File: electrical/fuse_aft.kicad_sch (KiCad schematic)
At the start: 4 parts, among them U1 GSU25, U2 GTX45R, U4 GSA 28 PITCH, U8 ESSENTIAL

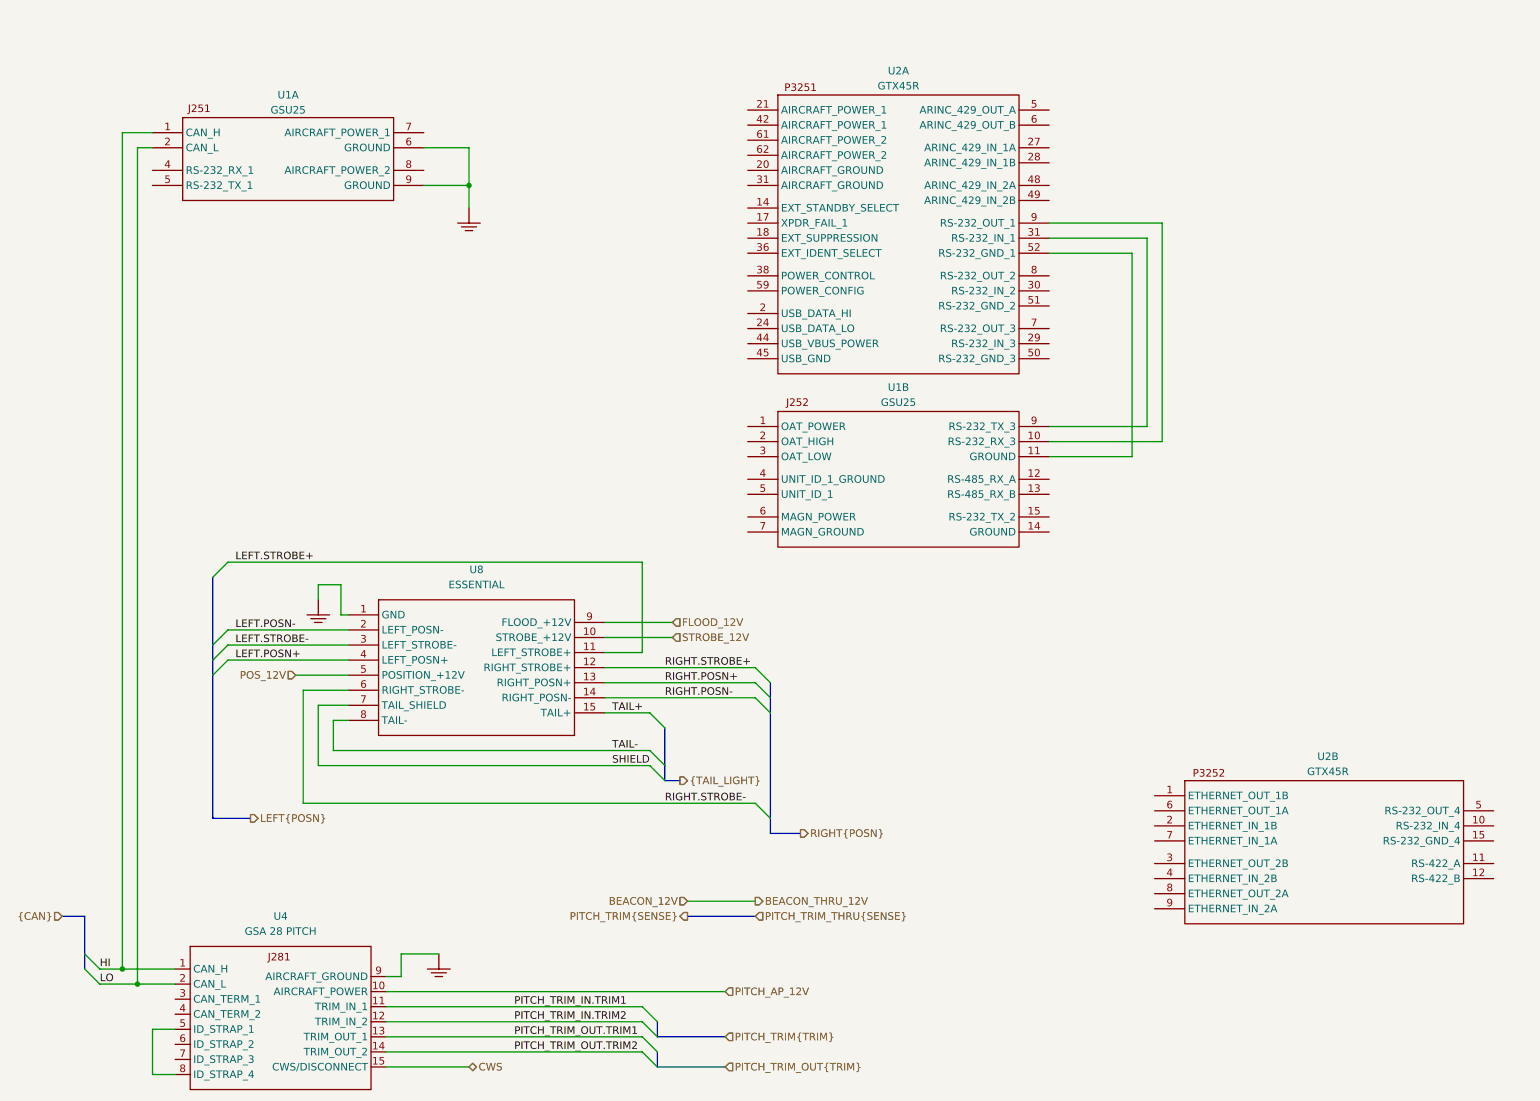
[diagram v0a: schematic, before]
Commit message: 🎮 Working on electrical schematic
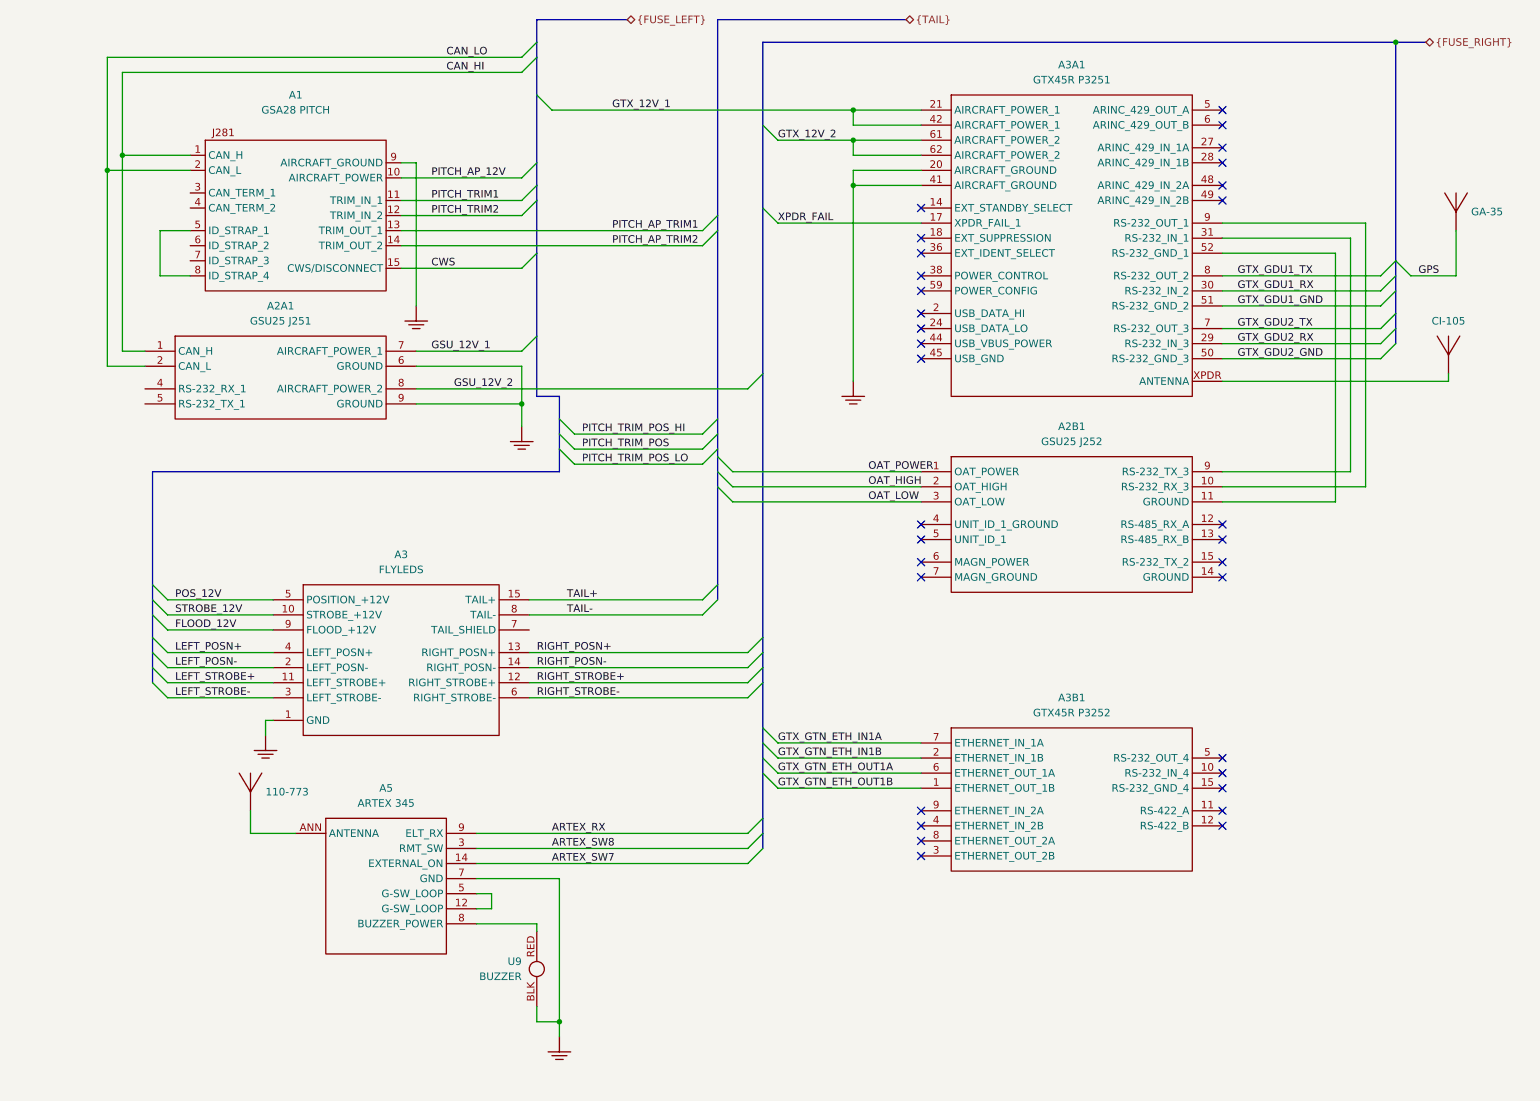
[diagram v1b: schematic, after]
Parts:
- removed U1: GSU25, symbol Garmin:GSU25
- removed U2: GTX45R, symbol Garmin:GTX45R
- removed U8: ESSENTIAL, symbol FlyLeds:ESSENTIAL_CONTROLLER
- added A2A1: GSU25 J251, symbol Garmin:GSU25_J251
- added A2B1: GSU25 J252, symbol Garmin:GSU25_J252
- added A3: FLYLEDS, symbol FlyLeds:ESSENTIAL_CONTROLLER
- added A3A1: GTX45R P3251, symbol Garmin:GTX45R_P3251
- added A3B1: GTX45R P3252, symbol Garmin:GTX45R_P3252
- added A5: ARTEX 345, symbol Misc:ARTEX345
- added A6: CI-105, symbol Misc:ANTENNA
- added A7: GA-35, symbol Misc:ANTENNA
- added A8: 110-773, symbol Misc:ANTENNA
- added U9: BUZZER, symbol Misc:BUZZER
- A1: renamed from U4; value GSA 28 PITCH -> GSA28 PITCH
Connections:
- net FLOOD_12V: now also A3.9 (FLOOD_+12V)
- net GND: now also A2A1.6 (GROUND), A2A1.9 (GROUND), A3.1 (GND), A3A1.20 (AIRCRAFT_GROUND), A3A1.41 (AIRCRAFT_GROUND), A5.7 (GND), U9.BLK
- net POS_12V: now also A3.5 (POSITION_+12V)
- net STROBE_12V: now also A3.10 (STROBE_+12V)
- net TAIL+: now also A3.15 (TAIL+)
- net TAIL-: now also A3.8 (TAIL-)
- net HI renamed CAN_HI
- net CAN_HI: now also A2A1.1 (CAN_H)
- net LO renamed CAN_LO
- net CAN_LO: now also A2A1.2 (CAN_L)
- net PITCH_TRIM_IN.TRIM1 renamed PITCH_TRIM1
- net PITCH_TRIM_IN.TRIM2 renamed PITCH_TRIM2
- net PITCH_TRIM_OUT.TRIM1 renamed PITCH_AP_TRIM1
- net PITCH_TRIM_OUT.TRIM2 renamed PITCH_AP_TRIM2
- new net: A3A1.XPDR (ANTENNA), A6. (SIGNAL)
- new net: A2B1.9 (RS-232_TX_3), A3A1.31 (RS-232_IN_1)
- new net: A2B1.11 (GROUND), A3A1.52 (RS-232_GND_1)
- new net: A2B1.10 (RS-232_RX_3), A3A1.9 (RS-232_OUT_1)
- new net: A5.12 (G-SW_LOOP), A5.5 (G-SW_LOOP)
- new net: A5.8 (BUZZER_POWER), U9.RED
- new net: A5.ANN (ANTENNA), A8. (SIGNAL)
- new net ARTEX_RX: A5.9 (ELT_RX)
- new net ARTEX_SW7: A5.14 (EXTERNAL_ON)
- new net ARTEX_SW8: A5.3 (RMT_SW)
- new net GPS: A7. (SIGNAL)
- new net GSU_12V_1: A2A1.7 (AIRCRAFT_POWER_1)
- new net GSU_12V_2: A2A1.8 (AIRCRAFT_POWER_2)
- new net GTX_12V_1: A3A1.21 (AIRCRAFT_POWER_1), A3A1.42 (AIRCRAFT_POWER_1)
- new net GTX_12V_2: A3A1.61 (AIRCRAFT_POWER_2), A3A1.62 (AIRCRAFT_POWER_2)
- new net GTX_GDU1_GND: A3A1.51 (RS-232_GND_2)
- new net GTX_GDU1_RX: A3A1.30 (RS-232_IN_2)
- new net GTX_GDU1_TX: A3A1.8 (RS-232_OUT_2)
- new net GTX_GDU2_GND: A3A1.50 (RS-232_GND_3)
- new net GTX_GDU2_RX: A3A1.29 (RS-232_IN_3)
- new net GTX_GDU2_TX: A3A1.7 (RS-232_OUT_3)
- new net GTX_GTN_ETH_IN1A: A3B1.7 (ETHERNET_IN_1A)
- new net GTX_GTN_ETH_IN1B: A3B1.2 (ETHERNET_IN_1B)
- new net GTX_GTN_ETH_OUT1A: A3B1.6 (ETHERNET_OUT_1A)
- new net GTX_GTN_ETH_OUT1B: A3B1.1 (ETHERNET_OUT_1B)
- new net LEFT_POSN+: A3.4 (LEFT_POSN+)
- new net LEFT_POSN-: A3.2 (LEFT_POSN-)
- new net LEFT_STROBE+: A3.11 (LEFT_STROBE+)
- new net LEFT_STROBE-: A3.3 (LEFT_STROBE-)
- new net OAT_HIGH: A2B1.2 (OAT_HIGH)
- new net OAT_LOW: A2B1.3 (OAT_LOW)
- new net OAT_POWER: A2B1.1 (OAT_POWER)
- new net RIGHT_POSN+: A3.13 (RIGHT_POSN+)
- new net RIGHT_POSN-: A3.14 (RIGHT_POSN-)
- new net RIGHT_STROBE+: A3.12 (RIGHT_STROBE+)
- new net RIGHT_STROBE-: A3.6 (RIGHT_STROBE-)
- new net XPDR_FAIL: A3A1.17 (XPDR_FAIL_1)
- no-connect marks 0 -> 32
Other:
- moved on the sheet: A1
